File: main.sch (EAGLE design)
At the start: 562 parts, among them CN1 50 PIN 0.5MM, CN2 10067847-001RLF, CN3 632723300011, CN4 FF0881SA1, CN5 15PIN 0.5MM, CN6 31 PIN FPC, Q1 2N7002, Q2 FDN302P, Q3 2N7002, Q5 SI7489DP, SW2 TACT, SW3 TACT, SW4 TACT, SW5 TACT, SW7 TACT, SW8 SLIDE SPDT, U1 GMAX0505-DV, U10 TPS70950, U11 FT601Q, U12 CBTU02043, U13 MAX25300B, U14 ESP32, U15 MAX25300B, U16 INA180, U17 AP62301, U18 AP62301, U19 SCHMITT, U2 XC7Z014S-1CLG484C, U20 MAX25300B, U21 NOT, U22 MAX25300B, U23 SN74LVC1G3, U24 NAND, U25 EMC1812T, U26 BIPOLAR HALL, U27 LM2663, U28 ADS7867, U29 LM2663, U3 IS43TR16128CL-125KBLI, U30 LM2731X, U31 USBLC6-2SC6, U32 MAX1735, U33 MP2148, U34 TPS22917, U35 AP62301, U36 TLV61046A, U37 W25Q128JV, U38 TPS70918, U39 AP62301, U4 AP63300WU-7, U5 STM32L431RBT, U6 USB ESD, U7 ACT2861QI301-T, U8 TPS70918, U9 STUSB4500

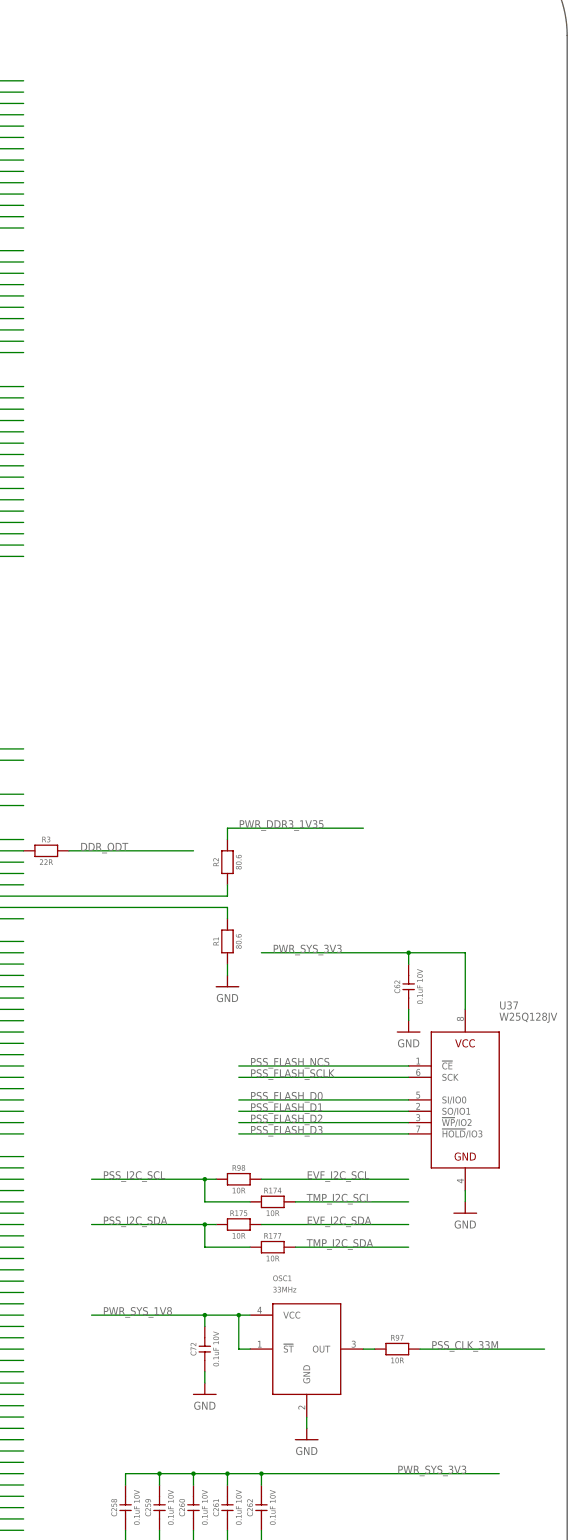
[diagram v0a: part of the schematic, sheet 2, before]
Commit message: DDR3 length matched
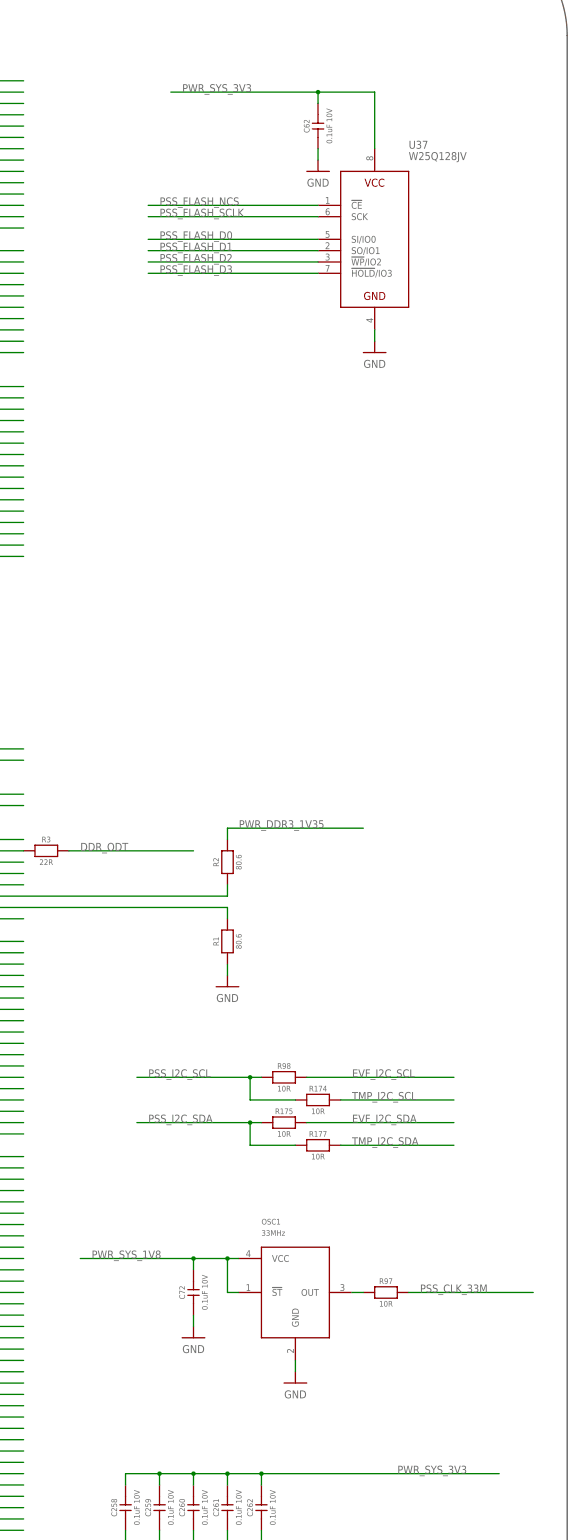
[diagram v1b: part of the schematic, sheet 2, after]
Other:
- moved on the sheet: C62, C72, OSC1, R174, R175, R177, R97, R98, U37
